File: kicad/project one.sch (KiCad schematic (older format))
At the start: 0 parts

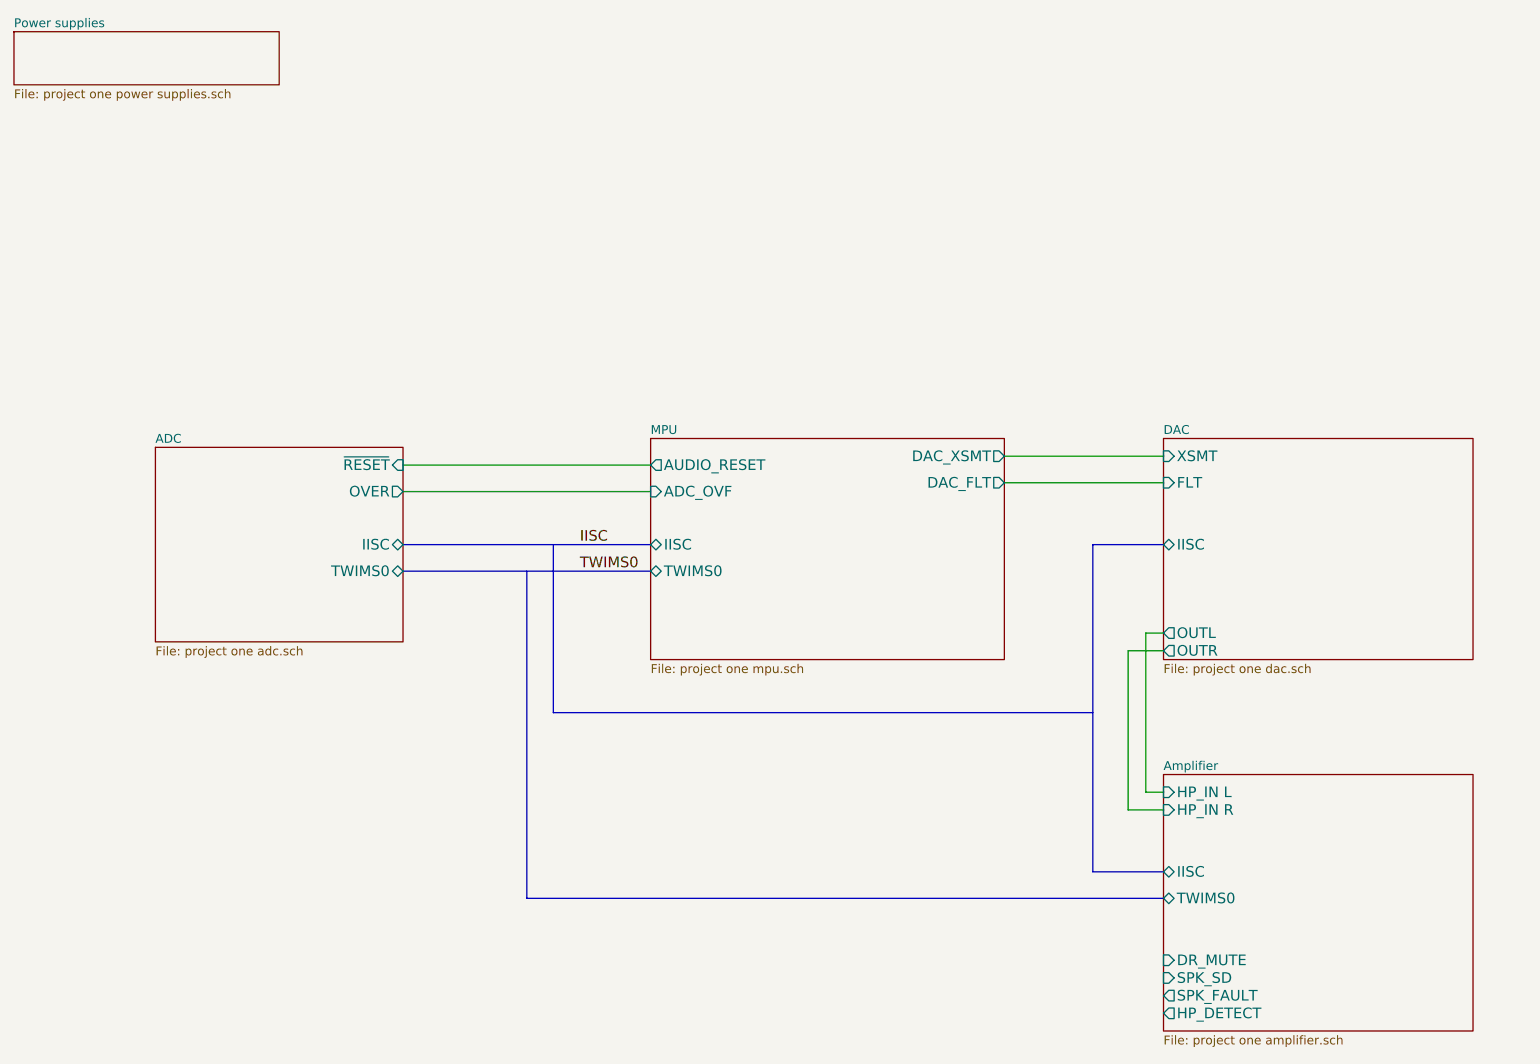
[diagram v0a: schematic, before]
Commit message: More stuff....
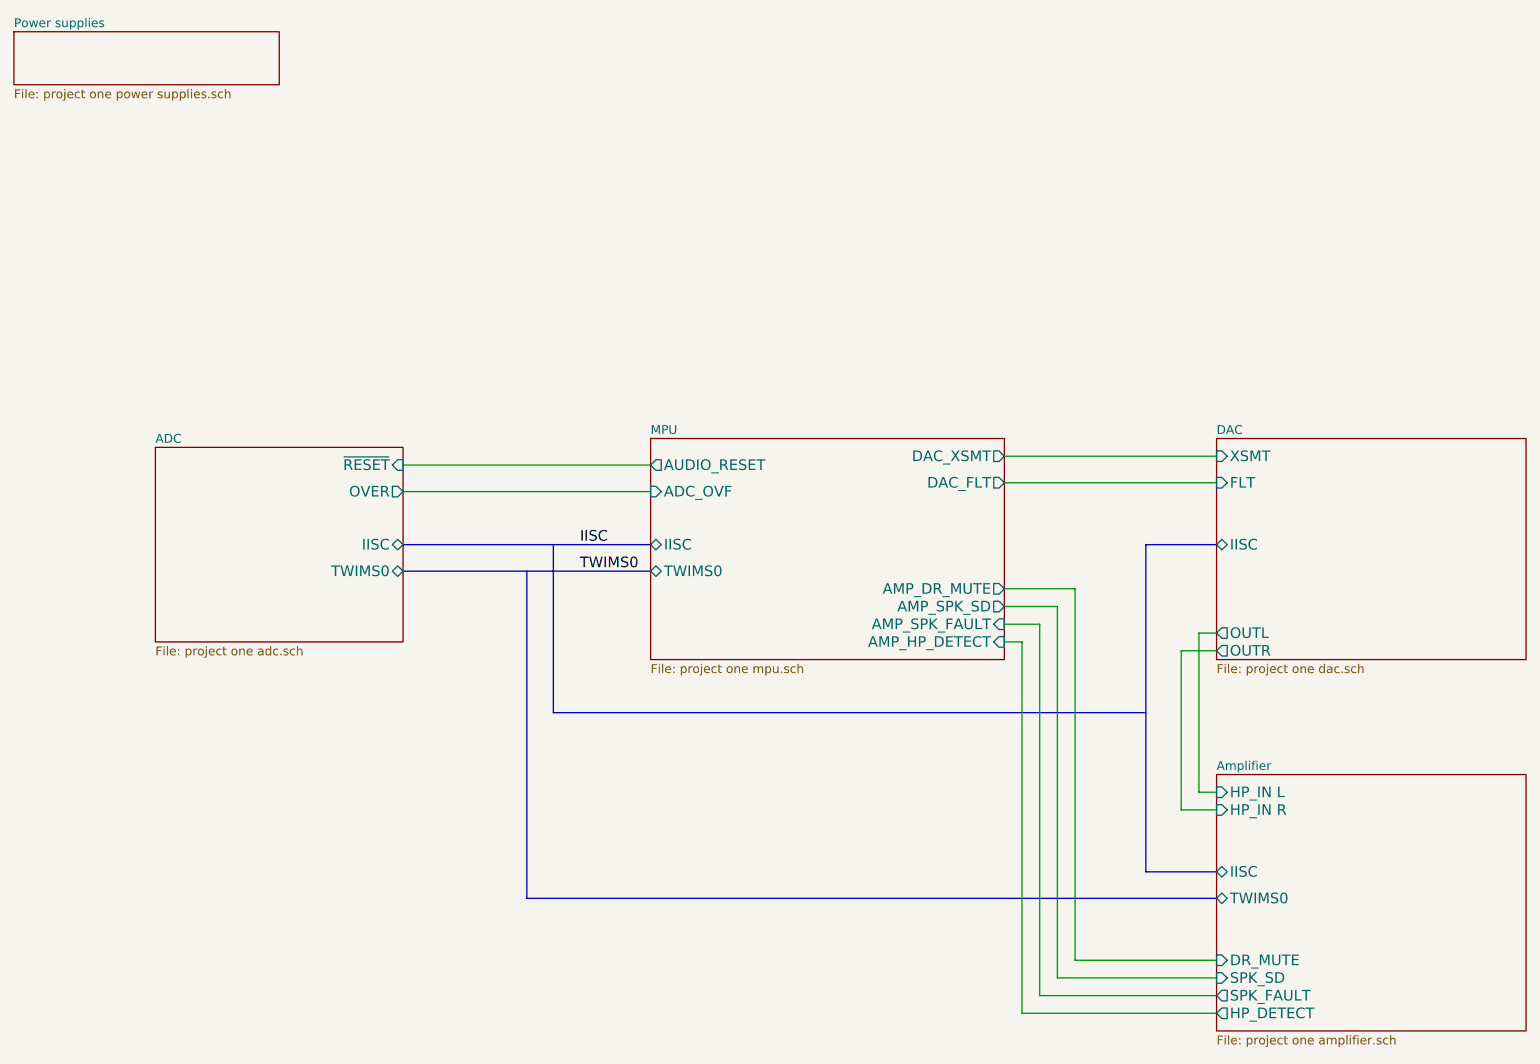
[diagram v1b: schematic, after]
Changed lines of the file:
@@
 Sheet 1 6
 Title "Project One"
-Date "6 may 2014"
+Date "9 may 2014"
 Rev "0.0.0"
 Comp "Ali Kocaturk"
@@
 $EndSheet
 $Sheet
+S 1400 3000 1400 1100
+U 536732E3
+F0 "ADC" 50
+F1 "project one adc.sch" 50
+F2 "IISC" B R 2800 3550 60
+F3 "TWIMS0" B R 2800 3700 60
+F4 "~RESET" I R 2800 3100 60
+F5 "OVER" O R 2800 3250 60
+$EndSheet
+Text Label 3800 3550 0    60   ~ 0
+IISC
+Text Label 3800 3700 0    60   ~ 0
+TWIMS0
+$Sheet
+S 7400 2950 1750 1250
+U 53675CA8
+F0 "DAC" 50
+F1 "project one dac.sch" 50
+F2 "OUTL" O L 7400 4050 60
+F3 "OUTR" O L 7400 4150 60
+F4 "FLT" I L 7400 3200 60
+F5 "XSMT" I L 7400 3050 60
+F6 "IISC" B L 7400 3550 60
+$EndSheet
+$Sheet
+S 7400 4850 1750 1450
+U 5367165F
+F0 "Amplifier" 50
+F1 "project one amplifier.sch" 50
+F2 "HP_DETECT" O L 7400 6200 60
+F3 "SPK_FAULT" O L 7400 6100 60
+F4 "SPK_SD" I L 7400 6000 60
+F5 "TWIMS0" B L 7400 5550 60
+F6 "IISC" B L 7400 5400 60
+F7 "DR_MUTE" I L 7400 5900 60
+F8 "HP_IN L" I L 7400 4950 60
+F9 "HP_IN R" I L 7400 5050 60
+$EndSheet
+$Sheet
 S 4200 2950 2000 1250
 U 5365F364
@@
 F6 "DAC_XSMT" O R 6200 3050 60
 F7 "DAC_FLT" O R 6200 3200 60
-$EndSheet
-$Sheet
-S 1400 3000 1400 1100
-U 536732E3
-F0 "ADC" 50
-F1 "project one adc.sch" 50
-F2 "IISC" B R 2800 3550 60
-F3 "TWIMS0" B R 2800 3700 60
-F4 "~RESET" I R 2800 3100 60
-F5 "OVER" O R 2800 3250 60
+F8 "AMP_SPK_FAULT" I R 6200 4000 60
+F9 "AMP_SPK_SD" O R 6200 3900 60
+F10 "AMP_DR_MUTE" O R 6200 3800 60
+F11 "AMP_HP_DETECT" I R 6200 4100 60
 $EndSheet
 Wire Bus Line
@@
 Wire Bus Line
 	2800 3700 4200 3700
-Text Label 3800 3550 0    60   ~ 0
-IISC
-Text Label 3800 3700 0    60   ~ 0
-TWIMS0
 Wire Wire Line
 	4200 3100 2800 3100
 Wire Wire Line
 	4200 3250 2800 3250
-$Sheet
-S 7100 2950 1750 1250
-U 53675CA8
-F0 "DAC" 50
-F1 "project one dac.sch" 50
-F2 "OUTL" O L 7100 4050 60
-F3 "OUTR" O L 7100 4150 60
-F4 "FLT" I L 7100 3200 60
-F5 "XSMT" I L 7100 3050 60
-F6 "IISC" B L 7100 3550 60
-$EndSheet
 Wire Bus Line
 	3650 3550 3650 4500
 Wire Bus Line
-	3650 4500 6700 4500
+	3650 4500 7000 4500
 Wire Bus Line
-	6700 3550 6700 5400
+	7000 3550 7000 5400
 Wire Bus Line
-	6700 3550 7100 3550
+	7000 3550 7400 3550
 Wire Wire Line
-	6200 3050 7100 3050
+	6200 3050 7400 3050
 Wire Wire Line
-	6200 3200 7100 3200
-$Sheet
-S 7100 4850 1750 1450
-U 5367165F
-F0 "Amplifier" 50
-F1 "project one amplifier.sch" 50
-F2 "HP_DETECT" O L 7100 6200 60
-F3 "SPK_FAULT" O L 7100 6100 60
-F4 "SPK_SD" I L 7100 6000 60
-F5 "TWIMS0" B L 7100 5550 60
-F6 "IISC" B L 7100 5400 60
-F7 "DR_MUTE" I L 7100 5900 60
-F8 "HP_IN L" I L 7100 4950 60
-F9 "HP_IN R" I L 7100 5050 60
-$EndSheet
+	6200 3200 7400 3200
 Wire Wire Line
-	7100 4950 7000 4950
+	7400 4950 7300 4950
 Wire Wire Line
-	7000 4950 7000 4050
+	7300 4950 7300 4050
 Wire Wire Line
-	7000 4050 7100 4050
+	7300 4050 7400 4050
 Wire Wire Line
-	7100 4150 6900 4150
+	7400 4150 7200 4150
 Wire Wire Line
-	6900 4150 6900 5050
+	7200 4150 7200 5050
 Wire Wire Line
-	6900 5050 7100 5050
+	7200 5050 7400 5050
 Wire Bus Line
-	6700 5400 7100 5400
+	7000 5400 7400 5400
 Wire Bus Line
-	7100 5550 3500 5550
+	7400 5550 3500 5550
 Wire Bus Line
 	3500 5550 3500 3700
+Wire Wire Line
+	6200 4100 6300 4100
+Wire Wire Line
+	6300 4100 6300 6200
+Wire Wire Line
+	6300 6200 7400 6200
+Wire Wire Line
+	7400 6100 6400 6100
+Wire Wire Line
+	6400 6100 6400 4000
+Wire Wire Line
+	6400 4000 6200 4000
+Wire Wire Line
+	6200 3900 6500 3900
+Wire Wire Line
+	6500 3900 6500 6000
+Wire Wire Line
+	6500 6000 7400 6000
+Wire Wire Line
+	7400 5900 6600 5900
+Wire Wire Line
+	6600 5900 6600 3800
+Wire Wire Line
+	6600 3800 6200 3800
 $EndSCHEMATC
